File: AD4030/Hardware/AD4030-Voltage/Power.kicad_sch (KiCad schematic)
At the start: 1 part, among them U501 TEC3-2419WI

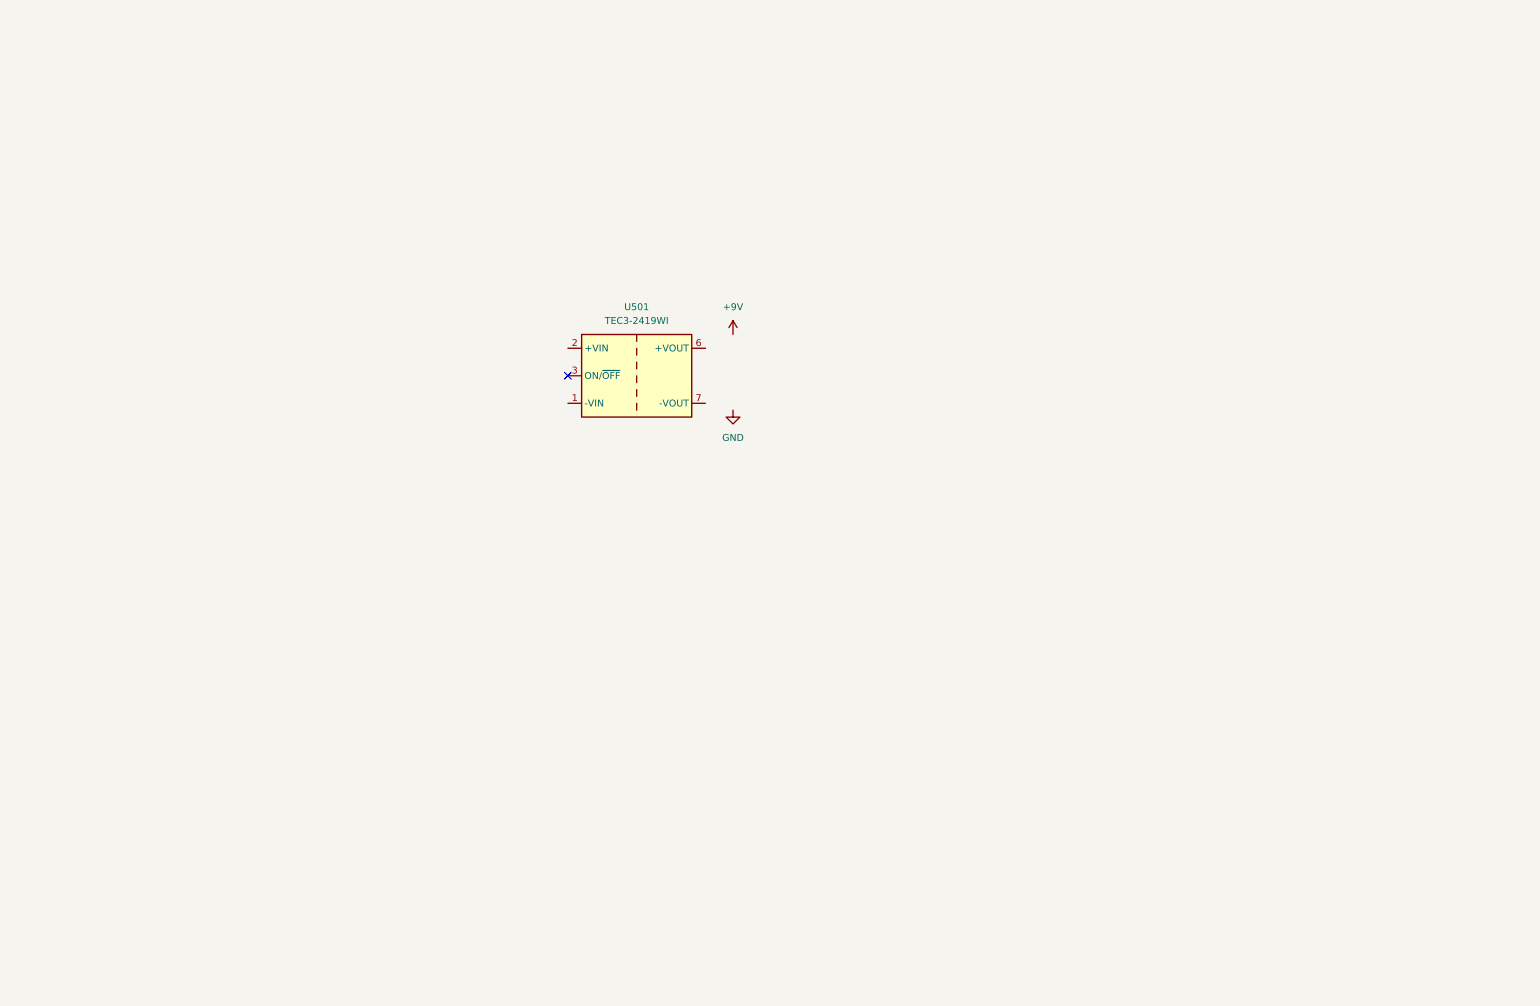
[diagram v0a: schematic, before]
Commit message: Hardware
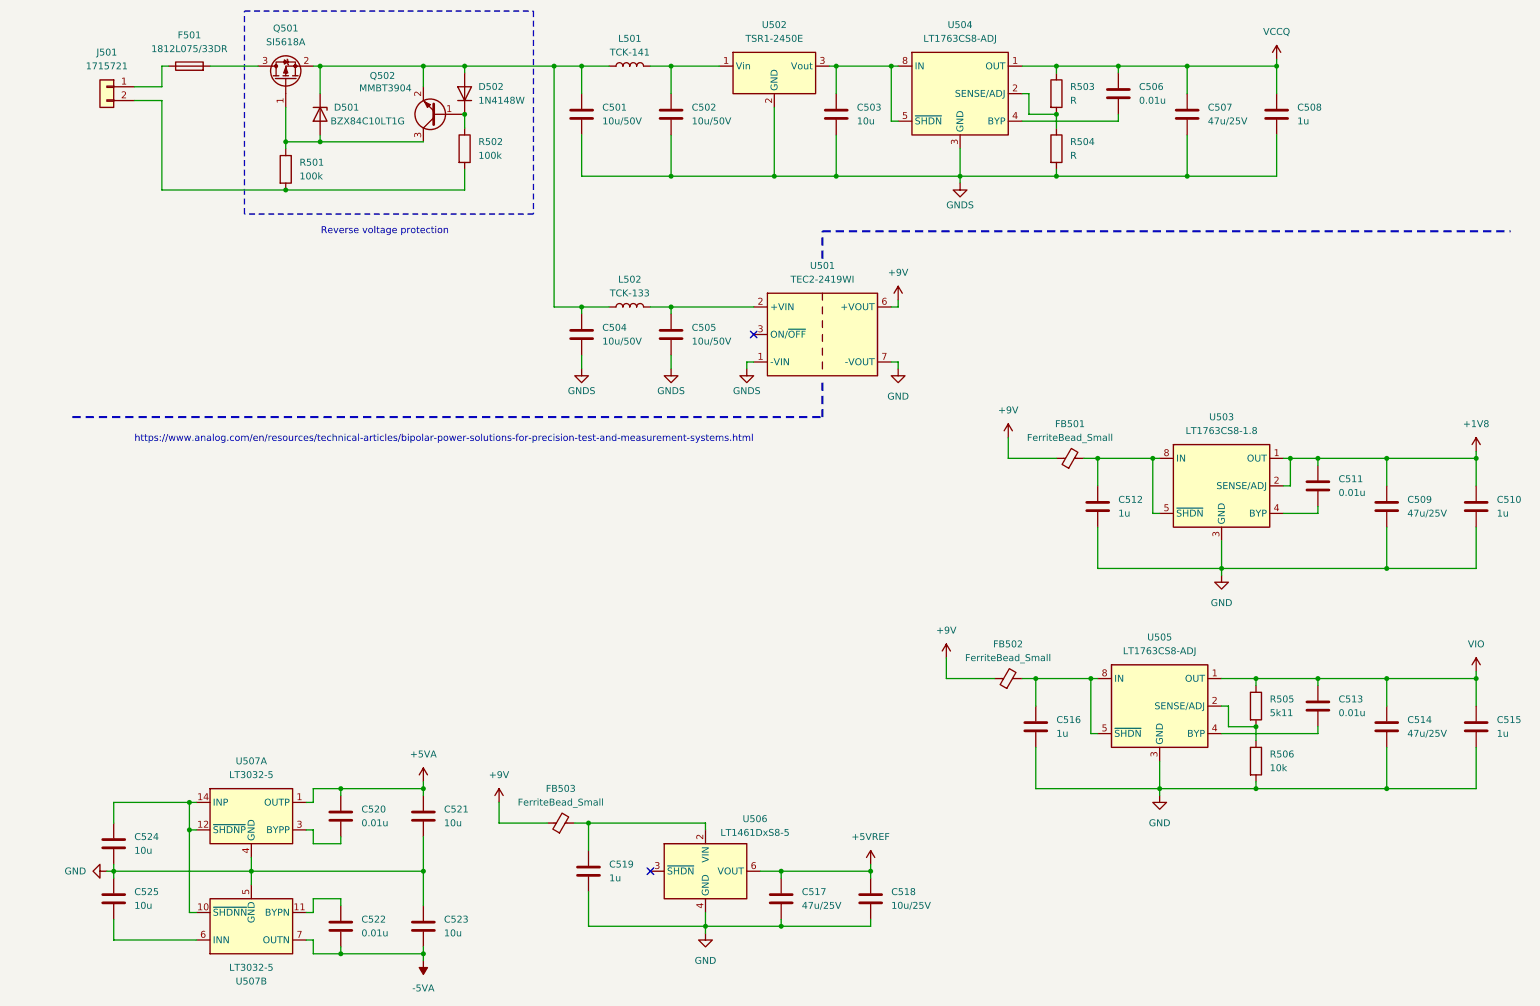
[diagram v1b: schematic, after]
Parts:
- added C501, C502, C504, C505: 10u/50V, symbol Device:C
- added C503, C521, C523, C524, C525: 10u, symbol Device:C
- added C506, C511, C513, C520, C522: 0.01u, symbol Device:C
- added C507, C509, C514, C517: 47u/25V, symbol Device:C
- added C508, C510, C512, C515, C516, C519: 1u, symbol Device:C
- added C518: 10u/25V, symbol Device:C
- added D501: BZX84C10LT1G, Package_TO_SOT_SMD:SOT-23, symbol Diode:BZX84Cxx
- added D502: 1N4148W, Diode_SMD:D_SOD-123, symbol Diode:1N4148W
- added F501: 1812L075/33DR, Fuse:Fuse_1812_4532Metric_Pad1.30x3.40mm_HandSolder, symbol Device:Fuse
- added FB501, FB502, FB503: FerriteBead_Small, symbol Device:FerriteBead_Small
- added J501: 1715721, TerminalBlock_Phoenix:TerminalBlock_Phoenix_MKDS-1,5-2_1x02_P5.00mm_Horizontal, symbol Connector_Generic:Conn_01x02
- added L501: TCK-141, symbol Device:L
- added L502: TCK-133, symbol Device:L
- added Q501: SI5618A, Package_TO_SOT_SMD:SOT-23, symbol Device:Q_PMOS_GSD
- added Q502: MMBT3904, Package_TO_SOT_SMD:SOT-23, symbol Transistor_BJT:MMBT3904
- added R501, R502: 100k, Resistor_SMD:R_0603_1608Metric_Pad0.98x0.95mm_HandSolder, symbol Device:R
- added R503, R504: R, symbol Device:R
- added R505: 5k11, symbol Device:R
- added R506: 10k, symbol Device:R
- added U502: TSR1-2450E, Converter_DCDC:Converter_DCDC_TRACO_TSR1-xxxxE_THT, symbol Regulator_Switching:TSR1-2450E
- added U503: LT1763CS8-1.8, Package_SO:SOIC-8_3.9x4.9mm_P1.27mm, symbol AD4030:LT1763CS8
- added U504, U505: LT1763CS8-ADJ, Package_SO:SOIC-8_3.9x4.9mm_P1.27mm, symbol AD4030:LT1763CS8
- added U506: LT1461DxS8-5, Package_SO:SOIC-8_3.9x4.9mm_P1.27mm, symbol Reference_Voltage:LT1461DxS8-5
- added U507: LT3032-5, Package_DFN_QFN:Linear_DE14MA, symbol Regulator_Linear:LT3032-5
- U501: value TEC3-2419WI -> TEC2-2419WI
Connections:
- net +9V: now also U501.6 (+VOUT), FB501.1, FB502.1, FB503.1
- net GND: now also U501.7 (-VOUT), C509.2, C510.2, C512.2, C514.2, C515.2, C516.2, C517.2, C518.2, C519.2, C521.2, C523.1, C524.2, C525.1, R506.2, U503.3 (GND), U503.6 (GND), U503.7 (GND), U505.3 (GND), U505.6 (GND), U505.7 (GND), U506.4 (GND), U507.4 (GND), U507.5 (GND)
- net GNDS: now reaches U501.1 (-VIN)
- net GNDS: now also C501.2, C502.2, C503.2, C504.2, C505.2, C507.2, C508.2, R504.2, U502.2 (GND), U504.3 (GND), U504.6 (GND), U504.7 (GND)
- net at U501.2 (+VIN): now also C505.1, L502.2
- new net: C516.1, FB502.2, U505.5 (~{SHDN}), U505.8 (IN)
- new net: R505.2, R506.1, U505.2 (SENSE/ADJ)
- new net: C513.2, U505.4 (BYP)
- new net: D502.1 (K), Q502.1 (B), R502.1
- new net: C501.1, C504.1, D501.3 (K), D502.2 (A), L501.1, L502.1, Q501.2 (S), Q502.2 (E)
- new net: C502.1, L501.2, U502.1 (Vin)
- new net: C511.2, U503.4 (BYP)
- new net: C512.1, FB501.2, U503.5 (~{SHDN}), U503.8 (IN)
- new net: R503.2, R504.1, U504.2 (SENSE/ADJ)
- new net: C522.1, U507.11 (BYPN)
- new net: C519.1, FB503.2, U506.2 (VIN)
- new net: D501.1 (A), Q501.1 (G), Q502.3 (C), R501.1
- new net: C506.2, U504.4 (BYP)
- new net: C503.1, U502.3 (Vout), U504.5 (~{SHDN}), U504.8 (IN)
- new net: F501.1, J501.1 (Pin_1)
- new net: F501.2, Q501.3 (D)
- new net: C524.1, U507.10 (~{SHDNN}), U507.12 (~{SHDNP}), U507.14 (INP)
- new net: J501.2 (Pin_2), R501.2, R502.2
- new net: C525.2, U507.6 (INN), U507.9 (INN)
- new net: C520.2, U507.3 (BYPP)
- new net +1V8: C509.1, C510.1, C511.1, U503.1 (OUT), U503.2 (SENSE/ADJ)
- new net +5VA: C520.1, C521.1, U507.1 (OUTP)
- new net +5VREF: C517.1, C518.1, U506.6 (VOUT)
- new net -5VA: C522.2, C523.2, U507.7 (OUTN)
- new net VCCQ: C506.1, C507.1, C508.1, R503.1, U504.1 (OUT)
- new net VIO: C513.1, C514.1, C515.1, R505.1, U505.1 (OUT)
- no-connect marks 1 -> 2
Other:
- note added: "Reverse voltage protection"
- note added: "https://www.analog.com/en/resources/technical-articles/bipolar-power-solutions-for-precision-test-and-measurement-systems.html"
- moved on the sheet: U501

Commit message: Hardware
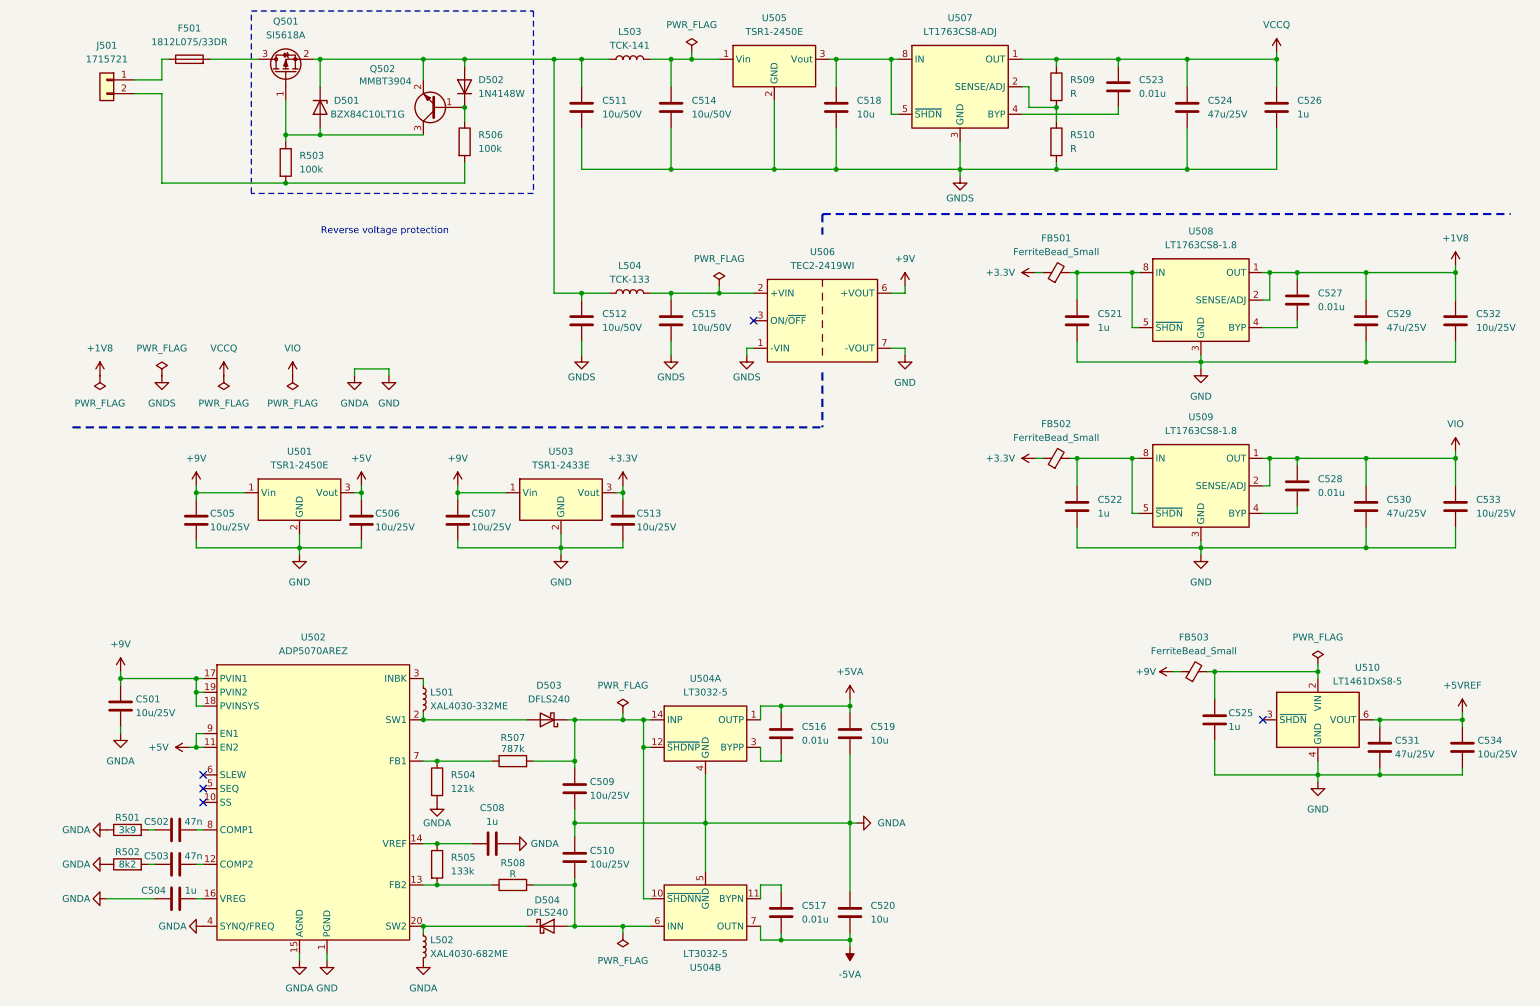
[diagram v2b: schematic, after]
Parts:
- removed C514: 47u/25V, symbol Device:C
- removed C516: 1u, symbol Device:C
- removed C524, C525: 10u, symbol Device:C
- removed L502: TCK-133, symbol Device:L
- removed R506: 10k, symbol Device:R
- removed U501: TEC2-2419WI, Converter_DCDC:Converter_DCDC_TRACO_TMR-xxxx_THT, symbol Converter_DCDC:TEC2-2419WI
- removed U505: LT1763CS8-ADJ, Package_SO:SOIC-8_3.9x4.9mm_P1.27mm, symbol AD4030:LT1763CS8
- added C501, C506, C507, C509, C510, C533: 10u/25V, Capacitor_SMD:C_1206_3216Metric_Pad1.33x1.80mm_HandSolder, symbol Device:C
- added C502, C503: 47n, Capacitor_SMD:C_0603_1608Metric_Pad1.08x0.95mm_HandSolder, symbol Device:C
- added C508: 1u, Capacitor_SMD:C_0603_1608Metric_Pad1.08x0.95mm_HandSolder, symbol Device:C
- added C512: 10u/50V, Capacitor_SMD:C_1210_3225Metric_Pad1.33x2.70mm_HandSolder, symbol Device:C
- added C522: 1u, Capacitor_SMD:C_0805_2012Metric_Pad1.18x1.45mm_HandSolder, symbol Device:C
- added C528: 0.01u, Capacitor_SMD:C_0603_1608Metric_Pad1.08x0.95mm_HandSolder, symbol Device:C
- added C530: 47u/25V, Capacitor_SMD:C_1210_3225Metric_Pad1.33x2.70mm_HandSolder, symbol Device:C
- added D503, D504: DFLS240, symbol Device:D_Schottky
- added L501: XAL4030-332ME, symbol Device:L_Small
- added L502: XAL4030-682ME, symbol Device:L_Small
- added L504: TCK-133, symbol Device:L
- added R501: 3k9, Resistor_SMD:R_0603_1608Metric_Pad0.98x0.95mm_HandSolder, symbol Device:R
- added R502: 8k2, Resistor_SMD:R_0603_1608Metric_Pad0.98x0.95mm_HandSolder, symbol Device:R
- added R504: 121k, Resistor_SMD:R_0603_1608Metric_Pad0.98x0.95mm_HandSolder, symbol Device:R
- added R507: 787k, Resistor_SMD:R_0603_1608Metric_Pad0.98x0.95mm_HandSolder, symbol Device:R
- added R508: R, Resistor_SMD:R_0603_1608Metric_Pad0.98x0.95mm_HandSolder, symbol Device:R
- added U501: TSR1-2450E, Converter_DCDC:Converter_DCDC_TRACO_TSR1-xxxxE_THT, symbol Regulator_Switching:TSR1-2450E
- added U502: ADP5070AREZ, Package_SO:ETSSOP-20-1EP_4.4x6.5mm_P0.65mm_EP3x4.2mm, symbol AD4030:ADP5070AREZ
- added U503: TSR1-2433E, Converter_DCDC:Converter_DCDC_TRACO_TSR1-xxxxE_THT, symbol Regulator_Switching:TSR1-2433E
- added U506: TEC2-2419WI, Converter_DCDC:Converter_DCDC_TRACO_TMR-xxxx_THT, symbol Converter_DCDC:TEC2-2419WI
- added U509: LT1763CS8-1.8, Package_SO:SOIC-8_3.9x4.9mm_P1.27mm, symbol AD4030:LT1763CS8
- C504: value 10u/50V -> 1u; footprint (none) -> Capacitor_SMD:C_0603_1608Metric_Pad1.08x0.95mm_HandSolder
- C505: value 10u/50V -> 10u/25V; footprint (none) -> Capacitor_SMD:C_1206_3216Metric_Pad1.33x1.80mm_HandSolder
- C511: renamed from C501; footprint (none) -> Capacitor_SMD:C_1210_3225Metric_Pad1.33x2.70mm_HandSolder
- C513: value 0.01u -> 10u/25V; footprint (none) -> Capacitor_SMD:C_1206_3216Metric_Pad1.33x1.80mm_HandSolder
- C514: renamed from C502; footprint (none) -> Capacitor_SMD:C_1210_3225Metric_Pad1.33x2.70mm_HandSolder
- C515: value 1u -> 10u/50V; footprint (none) -> Capacitor_SMD:C_1210_3225Metric_Pad1.33x2.70mm_HandSolder
- C516: renamed from C520; footprint (none) -> Capacitor_SMD:C_0603_1608Metric_Pad1.08x0.95mm_HandSolder
- C517: renamed from C522; footprint (none) -> Capacitor_SMD:C_0603_1608Metric_Pad1.08x0.95mm_HandSolder
- C518: renamed from C503; footprint (none) -> Capacitor_SMD:C_1206_3216Metric_Pad1.33x1.80mm_HandSolder
- C519: renamed from C521; footprint (none) -> Capacitor_SMD:C_1206_3216Metric_Pad1.33x1.80mm_HandSolder
- C520: renamed from C523; footprint (none) -> Capacitor_SMD:C_1206_3216Metric_Pad1.33x1.80mm_HandSolder
- C521: renamed from C512; footprint (none) -> Capacitor_SMD:C_0805_2012Metric_Pad1.18x1.45mm_HandSolder
- C523: renamed from C506; footprint (none) -> Capacitor_SMD:C_0603_1608Metric_Pad1.08x0.95mm_HandSolder
- C524: renamed from C507; footprint (none) -> Capacitor_SMD:C_1210_3225Metric_Pad1.33x2.70mm_HandSolder
- C525: renamed from C519; footprint (none) -> Capacitor_SMD:C_0805_2012Metric_Pad1.18x1.45mm_HandSolder
- C526: renamed from C508; footprint (none) -> Capacitor_SMD:C_0805_2012Metric_Pad1.18x1.45mm_HandSolder
- C527: renamed from C511; footprint (none) -> Capacitor_SMD:C_0603_1608Metric_Pad1.08x0.95mm_HandSolder
- C529: renamed from C509; footprint (none) -> Capacitor_SMD:C_1210_3225Metric_Pad1.33x2.70mm_HandSolder
- C531: renamed from C517; footprint (none) -> Capacitor_SMD:C_1210_3225Metric_Pad1.33x2.70mm_HandSolder
- C532: renamed from C510; value 1u -> 10u/25V; footprint (none) -> Capacitor_SMD:C_1206_3216Metric_Pad1.33x1.80mm_HandSolder
- C534: renamed from C518; footprint (none) -> Capacitor_SMD:C_1206_3216Metric_Pad1.33x1.80mm_HandSolder
- R505: value 5k11 -> 133k; footprint (none) -> Resistor_SMD:R_0603_1608Metric_Pad0.98x0.95mm_HandSolder
- R509: renamed from R503; footprint (none) -> Resistor_SMD:R_0603_1608Metric_Pad0.98x0.95mm_HandSolder
- R510: renamed from R504; footprint (none) -> Resistor_SMD:R_0603_1608Metric_Pad0.98x0.95mm_HandSolder
- renumbered L501 to L503, R501 to R503, R502 to R506, U507 to U504, U502 to U505, U504 to U507, U503 to U508, U506 to U510
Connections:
- net +9V: now also C505.1, C501.1, C507.1, U501.1 (Vin), U502.17 (PVIN1), U502.18 (PVINSYS), U502.19 (PVIN2), U503.1 (Vin), U506.6 (+VOUT); no longer FB501.1, FB502.1
- net GND: now also C504.1, C505.2, C513.2, C501.2, C506.2, C507.2, C508.2, C509.2, C510.1, C522.2, C530.2, C533.2, L502.2, R501.1, R502.1, R504.2, U501.2 (GND), U502.1 (PGND), U502.15 (AGND), U502.21 (EP), U502.4 (SYNQ/FREQ), U503.2 (GND), U506.7 (-VOUT), U509.3 (GND), U509.6 (GND), U509.7 (GND); no longer C515.2
- net GNDS: now also C515.2, C512.2, U506.1 (-VIN); no longer C504.2, C505.2
- net VIO: now also C528.1, C530.1, C533.1, U509.1 (OUT), U509.2 (SENSE/ADJ); no longer C513.1, C515.1, R505.1
- net at FB502.2: now also C522.1, U509.5 (~{SHDN}), U509.8 (IN)
- net at R505.2: now also R508.1, U502.13 (FB2)
- net at C511.1, D501.3 (K), D502.2 (A)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: now also C512.1, L504.1; no longer C504.1
- net at U504.10 (~{SHDNN}), U504.12 (~{SHDNP}), U504.14 (INP): now also C509.1, D503.1 (K), R507.2
- net at U504.6 (INN), U504.9 (INN): now also C510.2, D504.2 (A), R508.2
- new net: C503.1, R502.2
- new net: C503.2, U502.12 (COMP2)
- new net: C502.1, R501.2
- new net: D504.1 (K), L502.1, U502.20 (SW2)
- new net: C515.1, L504.2, U506.2 (+VIN)
- new net: D503.2 (A), L501.2, U502.2 (SW1)
- new net: C508.1, R505.1, U502.14 (VREF)
- new net: C504.2, U502.16 (VREG)
- new net: C528.2, U509.4 (BYP)
- new net: L501.1, U502.3 (INBK)
- new net: R504.1, R507.1, U502.7 (FB1)
- new net: C502.2, U502.8 (COMP1)
- new net +3.3V: C513.1, FB501.1, FB502.1, U503.3 (Vout)
- new net +5V: C506.1, U501.3 (Vout), U502.11 (EN2), U502.9 (EN1)
- no-connect marks 2 -> 5
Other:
- note removed: "https://www.analog.com/en/resources/technical-articles/bipolar-power-solutions-for-precision-test-and-measurement-systems.html"
- moved on the sheet: C511, C514, C516, C517, C518, C519, C520, C521, C523, C524, C525, C526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
